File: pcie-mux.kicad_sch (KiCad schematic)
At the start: 6 parts, among them Q5 DTC014T_SOT-416, U5 TMUXHS4212IRKSR

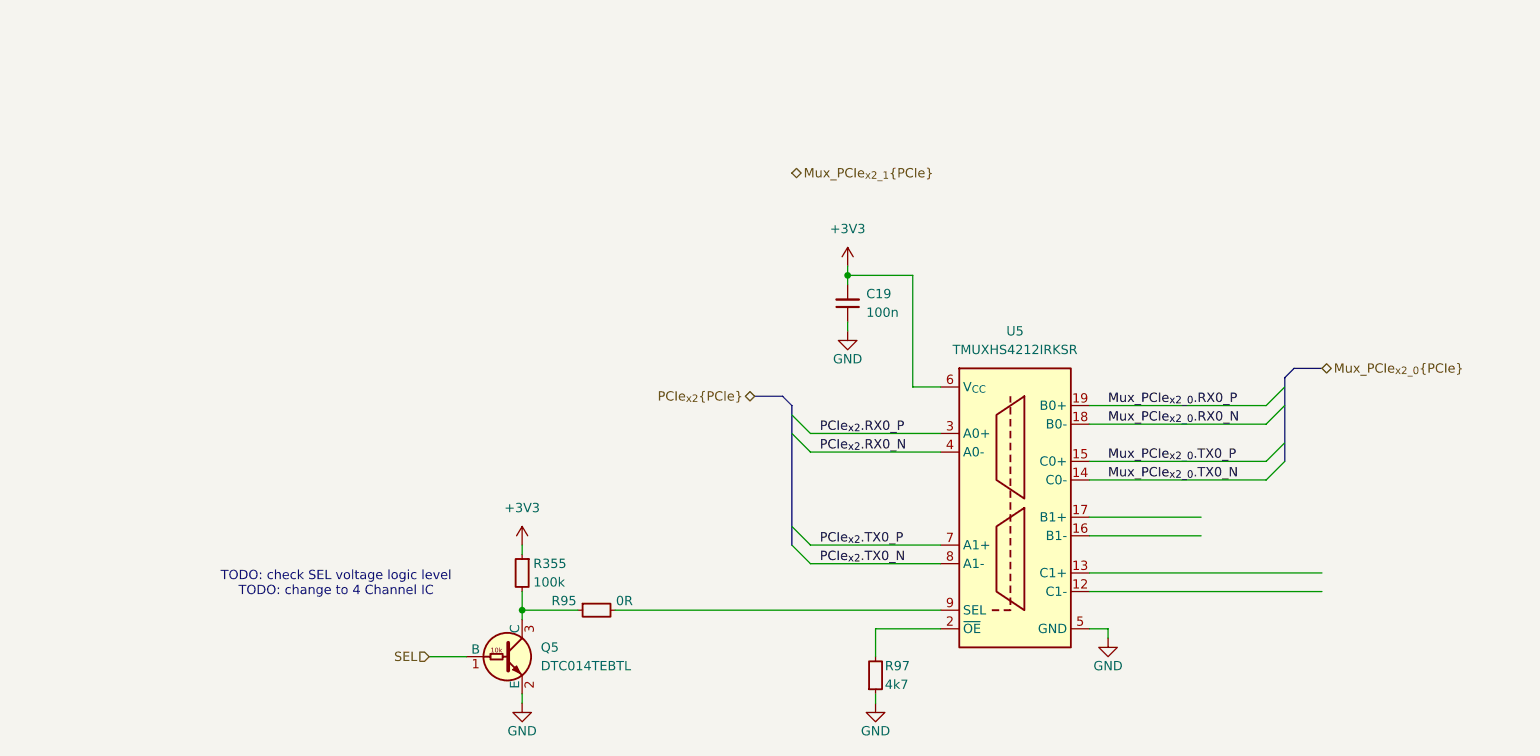
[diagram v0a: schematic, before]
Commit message: [#100765] Work on schematic
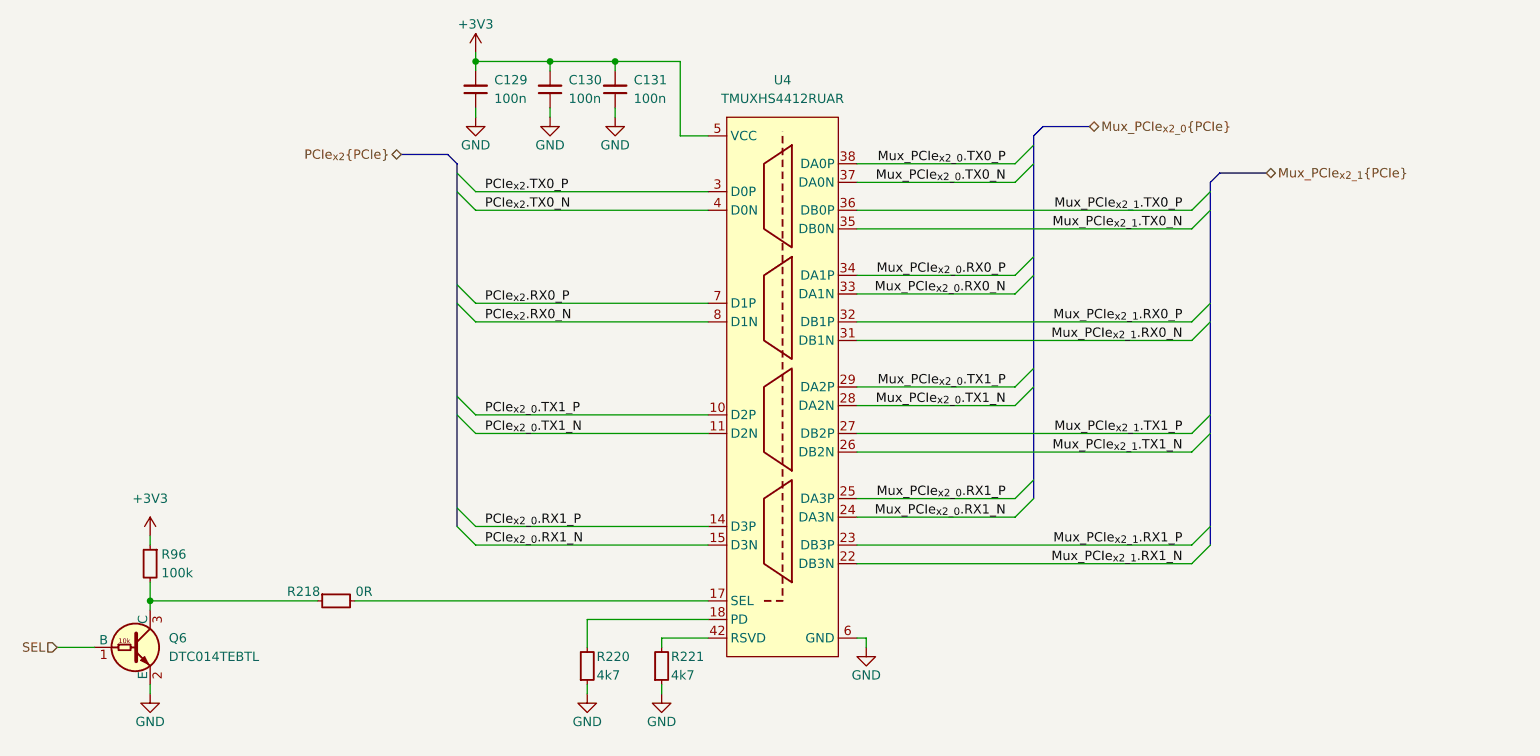
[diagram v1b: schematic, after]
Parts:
- removed C19: C_100n_0402, antmicro-footprints:C_0402_1005Metric, symbol antmicroCapacitors0402:C_100n_0402
- removed Q5: DTC014T_SOT-416, antmicro-footprints:SOT-416, symbol antmicroTransistorsBipolarSingle:DTC014T_SOT-416
- removed R355: R_100k_0402, antmicro-footprints:R_0402_1005Metric, symbol antmicroResistors0402:R_100k_0402
- removed R95: R_0R_0402, antmicro-footprints:R_0402_1005Metric, symbol antmicroResistors0402:R_0R_0402
- removed R97: R_4k7_0402, antmicro-footprints:R_0402_1005Metric, symbol antmicroResistors0402:R_4k7_0402
- removed U5: TMUXHS4212IRKSR, antmicro-footprints:VQFN-20_1EP_4.5x2.5mm_P0.5mm, symbol antmicroInterfaceAnalogSwitchesSpecialPurpose:TMUXHS4212IRKSR
- added C129, C130, C131: C_100n_0402, antmicro-footprints:C_0402_1005Metric, symbol antmicroCapacitors0402:C_100n_0402
- added Q6: DTC014T_SOT-416, antmicro-footprints:SOT-416, symbol antmicroTransistorsBipolarSingle:DTC014T_SOT-416
- added R218: R_0R_0402, antmicro-footprints:R_0402_1005Metric, symbol antmicroResistors0402:R_0R_0402
- added R220, R221: R_4k7_0402, antmicro-footprints:R_0402_1005Metric, symbol antmicroResistors0402:R_4k7_0402
- added R96: R_100k_0402, antmicro-footprints:R_0402_1005Metric, symbol antmicroResistors0402:R_100k_0402
- added U4: TMUXHS4412RUAR, antmicro-footprints:WQFN-42-1EP_3.5x9mm_P0.5mm, symbol antmicroInterfaceAnalogSwitchesSpecialPurpose:TMUXHS4412RUAR
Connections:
- net +3V3: now also C129.2, C130.2, C131.2, R96.1, U4.13 (VCC), U4.5 (VCC)
- net GND: now also C129.1, C130.1, C131.1, Q6.2 (E), R220.1, R221.1, U4.16 (GND), U4.21 (GND), U4.30 (GND), U4.39 (GND), U4.43 (GND), U4.6 (GND), U4.9 (GND)
- net Mux_PCIe_{x2_0}.RX0_N: now also U4.33 (DA1N)
- net Mux_PCIe_{x2_0}.RX0_P: now also U4.34 (DA1P)
- net Mux_PCIe_{x2_0}.TX0_N: now also U4.37 (DA0N)
- net Mux_PCIe_{x2_0}.TX0_P: now also U4.38 (DA0P)
- net PCIe_{x2}.RX0_N: now also U4.8 (D1N)
- net PCIe_{x2}.RX0_P: now also U4.7 (D1P)
- net PCIe_{x2}.TX0_N: now also U4.4 (D0N)
- net PCIe_{x2}.TX0_P: now also U4.3 (D0P)
- net SEL: now also Q6.1 (B)
- new net: Q6.3 (C), R218.1, R96.2
- new net: R218.2, U4.17 (SEL)
- new net: R221.2, U4.42 (RSVD)
- new net: R220.2, U4.18 (PD)
- new net Mux_PCIe_{x2_0}.RX1_N: U4.24 (DA3N)
- new net Mux_PCIe_{x2_0}.RX1_P: U4.25 (DA3P)
- new net Mux_PCIe_{x2_0}.TX1_N: U4.28 (DA2N)
- new net Mux_PCIe_{x2_0}.TX1_P: U4.29 (DA2P)
- new net Mux_PCIe_{x2_1}.RX0_N: U4.31 (DB1N)
- new net Mux_PCIe_{x2_1}.RX0_P: U4.32 (DB1P)
- new net Mux_PCIe_{x2_1}.RX1_N: U4.22 (DB3N)
- new net Mux_PCIe_{x2_1}.RX1_P: U4.23 (DB3P)
- new net Mux_PCIe_{x2_1}.TX0_N: U4.35 (DB0N)
- new net Mux_PCIe_{x2_1}.TX0_P: U4.36 (DB0P)
- new net Mux_PCIe_{x2_1}.TX1_N: U4.26 (DB2N)
- new net Mux_PCIe_{x2_1}.TX1_P: U4.27 (DB2P)
- new net PCIe_{x2_0}.RX1_N: U4.15 (D3N)
- new net PCIe_{x2_0}.RX1_P: U4.14 (D3P)
- new net PCIe_{x2_0}.TX1_N: U4.11 (D2N)
- new net PCIe_{x2_0}.TX1_P: U4.10 (D2P)
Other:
- note removed: "TODO: check SEL voltage logic level TODO: change to 4 Channel IC"
